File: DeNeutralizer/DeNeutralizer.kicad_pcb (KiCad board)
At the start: 2 copper layers, 27.9 x 72 mm, 18 parts, among them J1 Screw_Terminal_01x03, J2 Screw_Terminal_01x03, J3 Screw_Terminal_01x03, J4 Screw_Terminal_01x03, J7 Screw_Terminal_01x02, J8 Screw_Terminal_01x05, J9 Screw_Terminal_01x02, U1 PC817

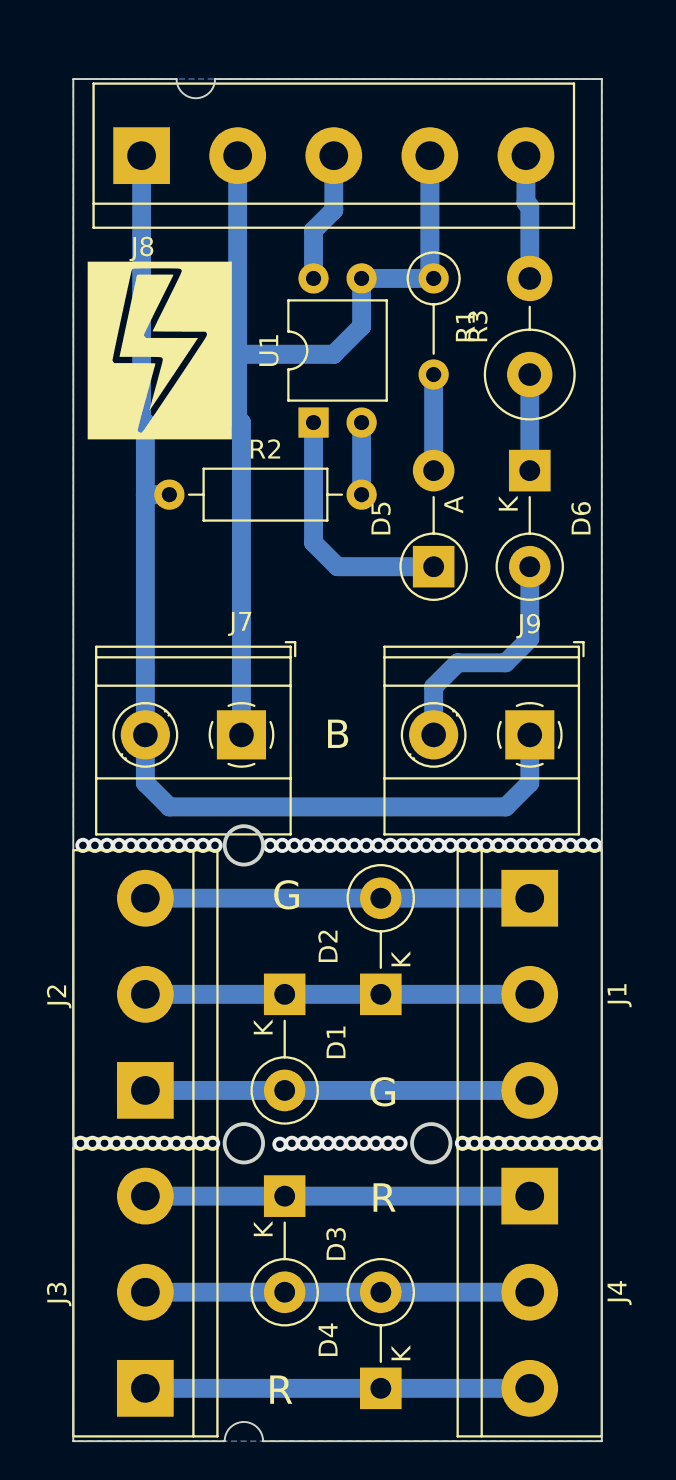
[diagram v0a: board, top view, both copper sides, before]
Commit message: Redesign the PCB
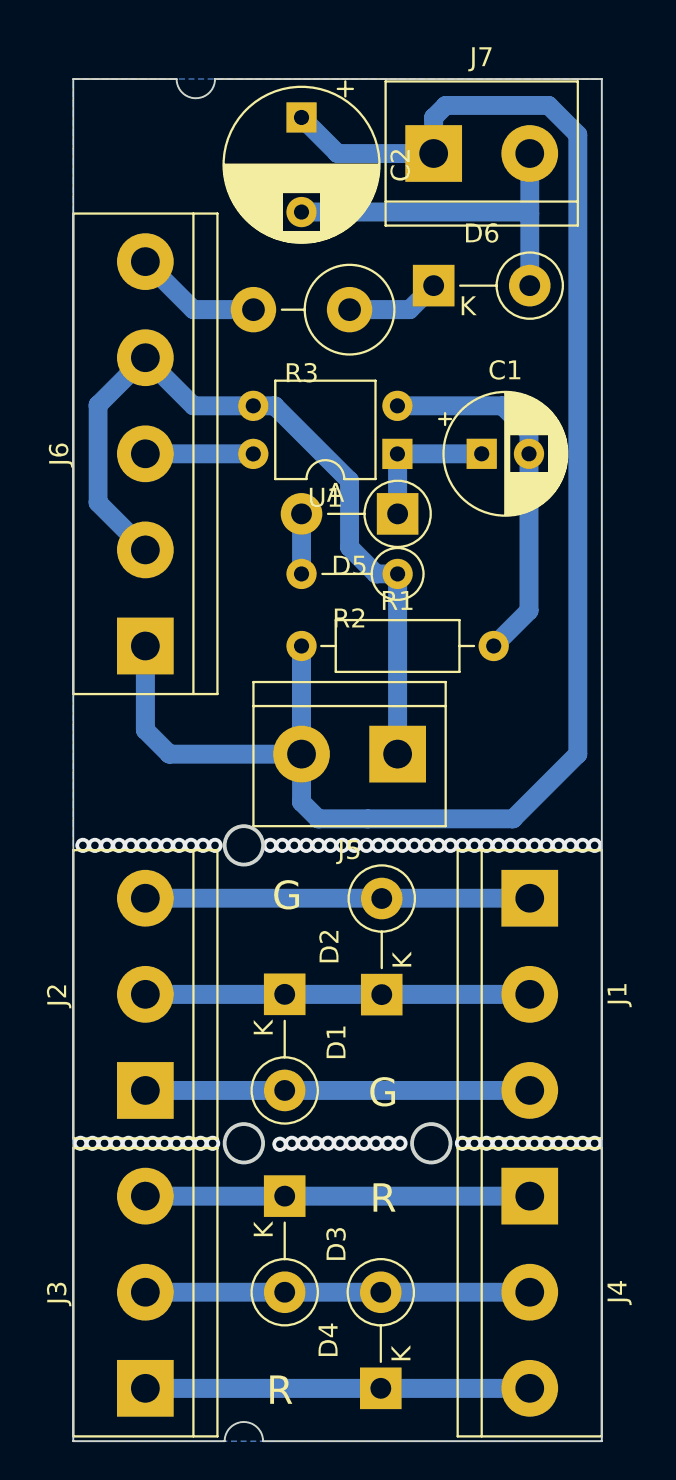
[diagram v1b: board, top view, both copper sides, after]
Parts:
- removed ?: LOGO, DeNeutralizer:Lightning
- removed J8: Screw_Terminal_01x05, TerminalBlock:TerminalBlock_bornier-5_P5.08mm
- removed J9: Screw_Terminal_01x02, TerminalBlock_Phoenix:TerminalBlock_Phoenix_MKDS-1,5-2-5.08_1x02_P5.08mm_Horizontal
- added C1: C_Polarized, Capacitor_THT:CP_Radial_D6.3mm_P2.50mm, F.Cu at (138.4, 88.3)
- added C2: C_Polarized, Capacitor_THT:CP_Radial_D8.0mm_P5.00mm, F.Cu at (128.9, 70.5)
- added J5: Screw_Terminal_01x02, TerminalBlock:TerminalBlock_bornier-2_P5.08mm, F.Cu at (134.0, 104.1)
- added J6: Screw_Terminal_01x05, TerminalBlock:TerminalBlock_bornier-5_P5.08mm, F.Cu at (120.7, 98.4)
- J7: footprint TerminalBlock_Phoenix:TerminalBlock_Phoenix_MKDS-1,5-2-5.08_1x02_P5.08mm_Horizontal -> TerminalBlock:TerminalBlock_bornier-2_P5.08mm
- R1: footprint Resistor_THT:R_Axial_DIN0414_L11.9mm_D4.5mm_P5.08mm_Vertical -> Resistor_THT:R_Axial_DIN0207_L6.3mm_D2.5mm_P10.16mm_Horizontal
- R2: footprint Resistor_THT:R_Axial_DIN0207_L6.3mm_D2.5mm_P10.16mm_Horizontal -> Resistor_THT:R_Axial_DIN0207_L6.3mm_D2.5mm_P5.08mm_Vertical
- R3: footprint Resistor_THT:R_Axial_DIN0207_L6.3mm_D2.5mm_P5.08mm_Vertical -> Resistor_THT:R_Axial_DIN0414_L11.9mm_D4.5mm_P5.08mm_Vertical
- moved J7 32.4 mm to (135.9, 72.4), turned to 0 degrees
- moved R1 18.7 mm to (128.9, 98.4), turned to 0 degrees
- moved R2 12.8 mm to (134.0, 94.6), turned to 180 degrees
- moved D6 11.0 mm to (135.9, 79.4), turned to 0 degrees
- moved R3 4.74 mm to (131.4, 80.6), turned to 180 degrees
- moved U1 4.73 mm to (134.0, 88.3), turned to 180 degrees
- moved D5 3.38 mm to (134.0, 91.4), turned to 180 degrees
- moved D2 0.05 mm to (133.1, 116.9)
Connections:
- D6 pad 2: Net-(J9-Pad2) -> Net-(C2-Pad2)
- J7 pad 1: Net-(J8-Pad2) -> Net-(C2-Pad1)
- J7 pad 2: Net-(J7-Pad2) -> Net-(C2-Pad2)
- R1 pad 1: Net-(D6-Pad1) -> Net-(C2-Pad1)
- R1 pad 2: Net-(J8-Pad5) -> Net-(C1-Pad2)
- R2 pad 1: Net-(J7-Pad2) -> Net-(J5-Pad1)
- R2 pad 2: Net-(C1-Pad2) -> Net-(D5-Pad2)
- R3 pad 1: Net-(J8-Pad2) -> Net-(D6-Pad1)
- R3 pad 2: Net-(D5-Pad2) -> Net-(J6-Pad5)
- U1 pad 3: Net-(J8-Pad2) -> Net-(J5-Pad1)
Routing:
- net Net-(C2-Pad1): track 0.00 -> 94.5 mm
- net Net-(J7-Pad2): track 58.4 -> 0.00 mm
- net Net-(J8-Pad2): track 51.1 -> 0.00 mm
- net Net-(J5-Pad1): track 0.00 -> 41.9 mm
- net Net-(C2-Pad2): track 0.00 -> 19.1 mm
- net Net-(C1-Pad2): track 3.81 -> 19.6 mm
- net Net-(J9-Pad2): track 12.5 -> 0.00 mm
- net Net-(J6-Pad5): track 0.00 -> 6.77 mm
- net Net-(J8-Pad5): track 6.57 -> 0.00 mm
- net Net-(C1-Pad1): track 13.2 -> 7.63 mm
- net Net-(D5-Pad2): track 5.08 -> 3.17 mm
- net Net-(J6-Pad3): track 6.93 -> 5.71 mm
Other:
- board text removed: "B"
